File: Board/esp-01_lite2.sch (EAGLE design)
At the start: 26 parts, among them IC1 TINY13-20SU, K1 setup, K2 reset, X1 235-102, X2 235-102

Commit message: LED works, server ok, ESP 24h
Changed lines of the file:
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@@
 <grid distance="10" unitdist="mil" unit="mil" style="lines" multiple="1" display="no" altdistance="0.01" altunitdist="inch" altunit="inch"/>
 <layers>
-<layer number="1" name="Top" color="4" fill="1" visible="no" active="no"/>
-<layer number="2" name="Route2" color="1" fill="3" visible="no" active="no"/>
-<layer number="3" name="Route3" color="4" fill="3" visible="no" active="no"/>
-<layer number="4" name="Route4" color="1" fill="4" visible="no" active="no"/>
-<layer number="5" name="Route5" color="4" fill="4" visible="no" active="no"/>
-<layer number="6" name="Route6" color="1" fill="8" visible="no" active="no"/>
-<layer number="7" name="Route7" color="4" fill="8" visible="no" active="no"/>
-<layer number="8" name="Route8" color="1" fill="2" visible="no" active="no"/>
-<layer number="9" name="Route9" color="4" fill="2" visible="no" active="no"/>
-<layer number="10" name="Route10" color="1" fill="7" visible="no" active="no"/>
-<layer number="11" name="Route11" color="4" fill="7" visible="no" active="no"/>
-<layer number="12" name="Route12" color="1" fill="5" visible="no" active="no"/>
-<layer number="13" name="Route13" color="4" fill="5" visible="no" active="no"/>
-<layer number="14" name="Route14" color="1" fill="6" visible="no" active="no"/>
-<layer number="15" name="Route15" color="4" fill="6" visible="no" active="no"/>
-<layer number="16" name="Bottom" color="1" fill="1" visible="no" active="no"/>
-<layer number="17" name="Pads" color="2" fill="1" visible="no" active="no"/>
-<layer number="18" name="Vias" color="2" fill="1" visible="no" active="no"/>
-<layer number="19" name="Unrouted" color="6" fill="1" visible="no" active="no"/>
-<layer number="20" name="Dimension" color="15" fill="1" visible="no" active="no"/>
-<layer number="21" name="tPlace" color="7" fill="1" visible="no" active="no"/>
-<layer number="22" name="bPlace" color="7" fill="1" visible="no" active="no"/>
-<layer number="23" name="tOrigins" color="15" fill="1" visible="no" active="no"/>
-<layer number="24" name="bOrigins" color="15" fill="1" visible="no" active="no"/>
-<layer number="25" name="tNames" color="7" fill="1" visible="no" active="no"/>
-<layer number="26" name="bNames" color="7" fill="1" visible="no" active="no"/>
-<layer number="27" name="tValues" color="7" fill="1" visible="no" active="no"/>
-<layer number="28" name="bValues" color="7" fill="1" visible="no" active="no"/>
+<layer number="1" name="Top" color="4" fill="1" visible="yes" active="no"/>
+<layer number="2" name="Route2" color="1" fill="3" visible="yes" active="no"/>
+<layer number="3" name="Route3" color="4" fill="3" visible="yes" active="no"/>
+<layer number="4" name="Route4" color="1" fill="4" visible="yes" active="no"/>
+<layer number="5" name="Route5" color="4" fill="4" visible="yes" active="no"/>
+<layer number="6" name="Route6" color="1" fill="8" visible="yes" active="no"/>
+<layer number="7" name="Route7" color="4" fill="8" visible="yes" active="no"/>
+<layer number="8" name="Route8" color="1" fill="2" visible="yes" active="no"/>
+<layer number="9" name="Route9" color="4" fill="2" visible="yes" active="no"/>
+<layer number="10" name="Route10" color="1" fill="7" visible="yes" active="no"/>
+<layer number="11" name="Route11" color="4" fill="7" visible="yes" active="no"/>
+<layer number="12" name="Route12" color="1" fill="5" visible="yes" active="no"/>
+<layer number="13" name="Route13" color="4" fill="5" visible="yes" active="no"/>
+<layer number="14" name="Route14" color="1" fill="6" visible="yes" active="no"/>
+<layer number="15" name="Route15" color="4" fill="6" visible="yes" active="no"/>
+<layer number="16" name="Bottom" color="1" fill="1" visible="yes" active="no"/>
+<layer number="17" name="Pads" color="2" fill="1" visible="yes" active="no"/>
+<layer number="18" name="Vias" color="2" fill="1" visible="yes" active="no"/>
+<layer number="19" name="Unrouted" color="6" fill="1" visible="yes" active="no"/>
+<layer number="20" name="Dimension" color="15" fill="1" visible="yes" active="no"/>
+<layer number="21" name="tPlace" color="7" fill="1" visible="yes" active="no"/>
+<layer number="22" name="bPlace" color="7" fill="1" visible="yes" active="no"/>
+<layer number="23" name="tOrigins" color="15" fill="1" visible="yes" active="no"/>
+<layer number="24" name="bOrigins" color="15" fill="1" visible="yes" active="no"/>
+<layer number="25" name="tNames" color="7" fill="1" visible="yes" active="no"/>
+<layer number="26" name="bNames" color="7" fill="1" visible="yes" active="no"/>
+<layer number="27" name="tValues" color="7" fill="1" visible="yes" active="no"/>
+<layer number="28" name="bValues" color="7" fill="1" visible="yes" active="no"/>
 <layer number="29" name="tStop" color="7" fill="3" visible="no" active="no"/>
 <layer number="30" name="bStop" color="7" fill="6" visible="no" active="no"/>
@@
 <layer number="35" name="tGlue" color="7" fill="4" visible="no" active="no"/>
 <layer number="36" name="bGlue" color="7" fill="5" visible="no" active="no"/>
-<layer number="37" name="tTest" color="7" fill="1" visible="no" active="no"/>
-<layer number="38" name="bTest" color="7" fill="1" visible="no" active="no"/>
+<layer number="37" name="tTest" color="7" fill="1" visible="yes" active="no"/>
+<layer number="38" name="bTest" color="7" fill="1" visible="yes" active="no"/>
 <layer number="39" name="tKeepout" color="4" fill="11" visible="no" active="no"/>
 <layer number="40" name="bKeepout" color="1" fill="11" visible="no" active="no"/>
@@
 <layer number="44" name="Drills" color="7" fill="1" visible="no" active="no"/>
 <layer number="45" name="Holes" color="7" fill="1" visible="no" active="no"/>
-<layer number="46" name="Milling" color="3" fill="1" visible="no" active="no"/>
-<layer number="47" name="Measures" color="7" fill="1" visible="no" active="no"/>
-<layer number="48" name="Document" color="7" fill="1" visible="no" active="no"/>
-<layer number="49" name="Reference" color="7" fill="1" visible="no" active="no"/>
-<layer number="50" name="dxf" color="7" fill="1" visible="no" active="no"/>
-<layer number="51" name="tDocu" color="7" fill="1" visible="no" active="no"/>
-<layer number="52" name="bDocu" color="7" fill="1" visible="no" active="no"/>
-<layer number="53" name="tGND_GNDA" color="7" fill="9" visible="no" active="no"/>
-<layer number="54" name="bGND_GNDA" color="1" fill="9" visible="no" active="no"/>
-<layer number="56" name="wert" color="7" fill="1" visible="no" active="no"/>
-<layer number="57" name="tCAD" color="7" fill="1" visible="no" active="no"/>
+<layer number="46" name="Milling" color="3" fill="1" visible="yes" active="no"/>
+<layer number="47" name="Measures" color="7" fill="1" visible="yes" active="no"/>
+<layer number="48" name="Document" color="7" fill="1" visible="yes" active="no"/>
+<layer number="49" name="Reference" color="7" fill="1" visible="yes" active="no"/>
+<layer number="50" name="dxf" color="7" fill="1" visible="yes" active="no"/>
+<layer number="51" name="tDocu" color="7" fill="1" visible="yes" active="no"/>
+<layer number="52" name="bDocu" color="7" fill="1" visible="yes" active="no"/>
+<layer number="53" name="tGND_GNDA" color="7" fill="9" visible="yes" active="no"/>
+<layer number="54" name="bGND_GNDA" color="1" fill="9" visible="yes" active="no"/>
+<layer number="56" name="wert" color="7" fill="1" visible="yes" active="no"/>
+<layer number="57" name="tCAD" color="7" fill="1" visible="yes" active="no"/>
 <layer number="90" name="Modules" color="5" fill="1" visible="yes" active="yes"/>
 <layer number="91" name="Nets" color="2" fill="1" visible="yes" active="yes"/>
@@
 <attribute name="VALUE" x="140.208" y="110.49" size="1.778" layer="96" rot="R180"/>
 </instance>
-<instance part="SJ1" gate="1" x="61.214" y="30.734" rot="R180"/>
+<instance part="SJ1" gate="1" x="61.214" y="30.734" smashed="yes" rot="R180">
+<attribute name="NAME" x="63.754" y="28.194" size="1.778" layer="95" rot="R180"/>
+<attribute name="VALUE" x="63.754" y="34.544" size="1.778" layer="96" rot="R180"/>
+</instance>
 <instance part="GND4" gate="1" x="66.294" y="23.114" smashed="yes">
 <attribute name="VALUE" x="63.754" y="20.574" size="1.778" layer="96"/>

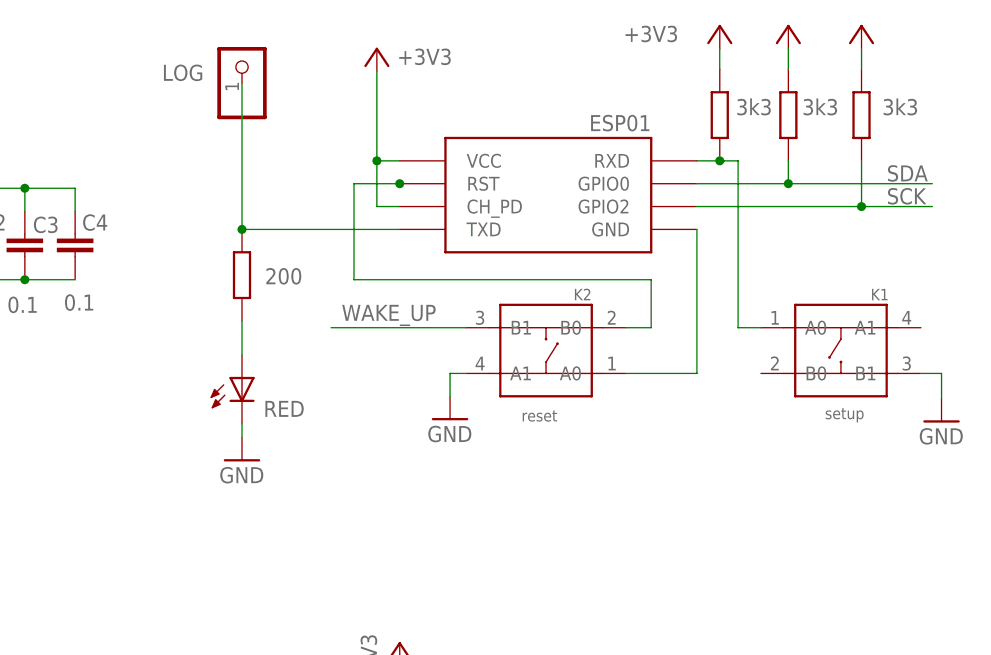
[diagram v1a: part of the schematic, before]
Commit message: new board
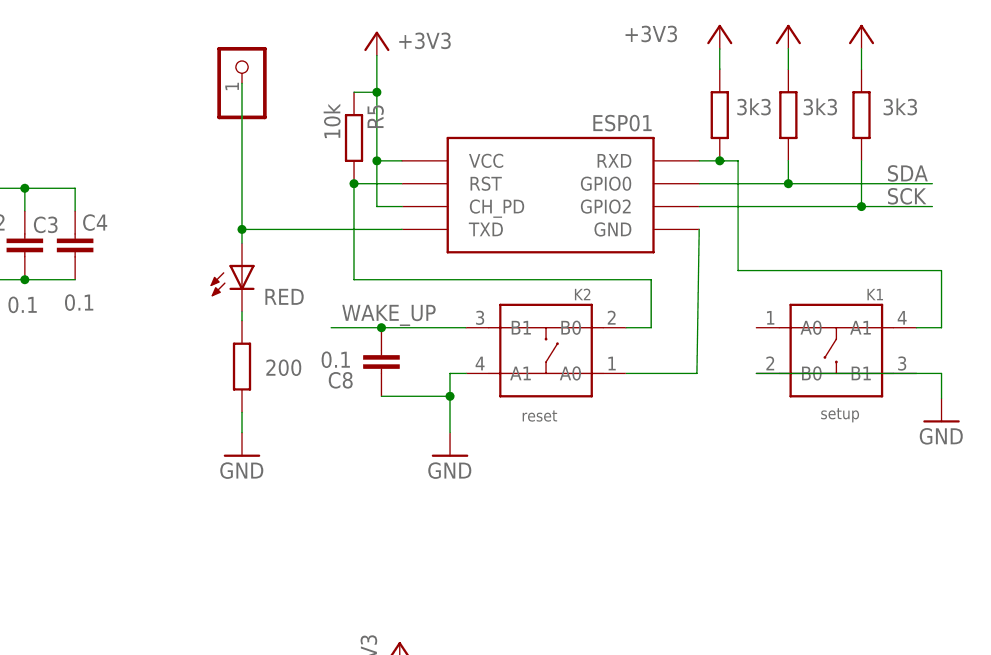
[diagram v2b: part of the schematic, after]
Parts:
- added C8: 0.1, resistor:C-EUC0805
- added R5: 10k, rcl:R-EU_R0805
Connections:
- removed net LOG: LOG.1, R4.1, U$1.TXD
- removed net N$12: LED1.A, R4.2
- new net N$1: LED1.A, LOG.1, U$1.TXD
- new net N$6: LED1.C, R4.1
- net +3V3: now also R5.1
- net GND: now also C8.1, K1.B0, R4.2; no longer LED1.C
- net N$2: now also R5.2
- net RX: now also K1.A1; no longer K1.A0
- net WAKE_UP: now also C8.2
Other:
- moved on the sheet: K1

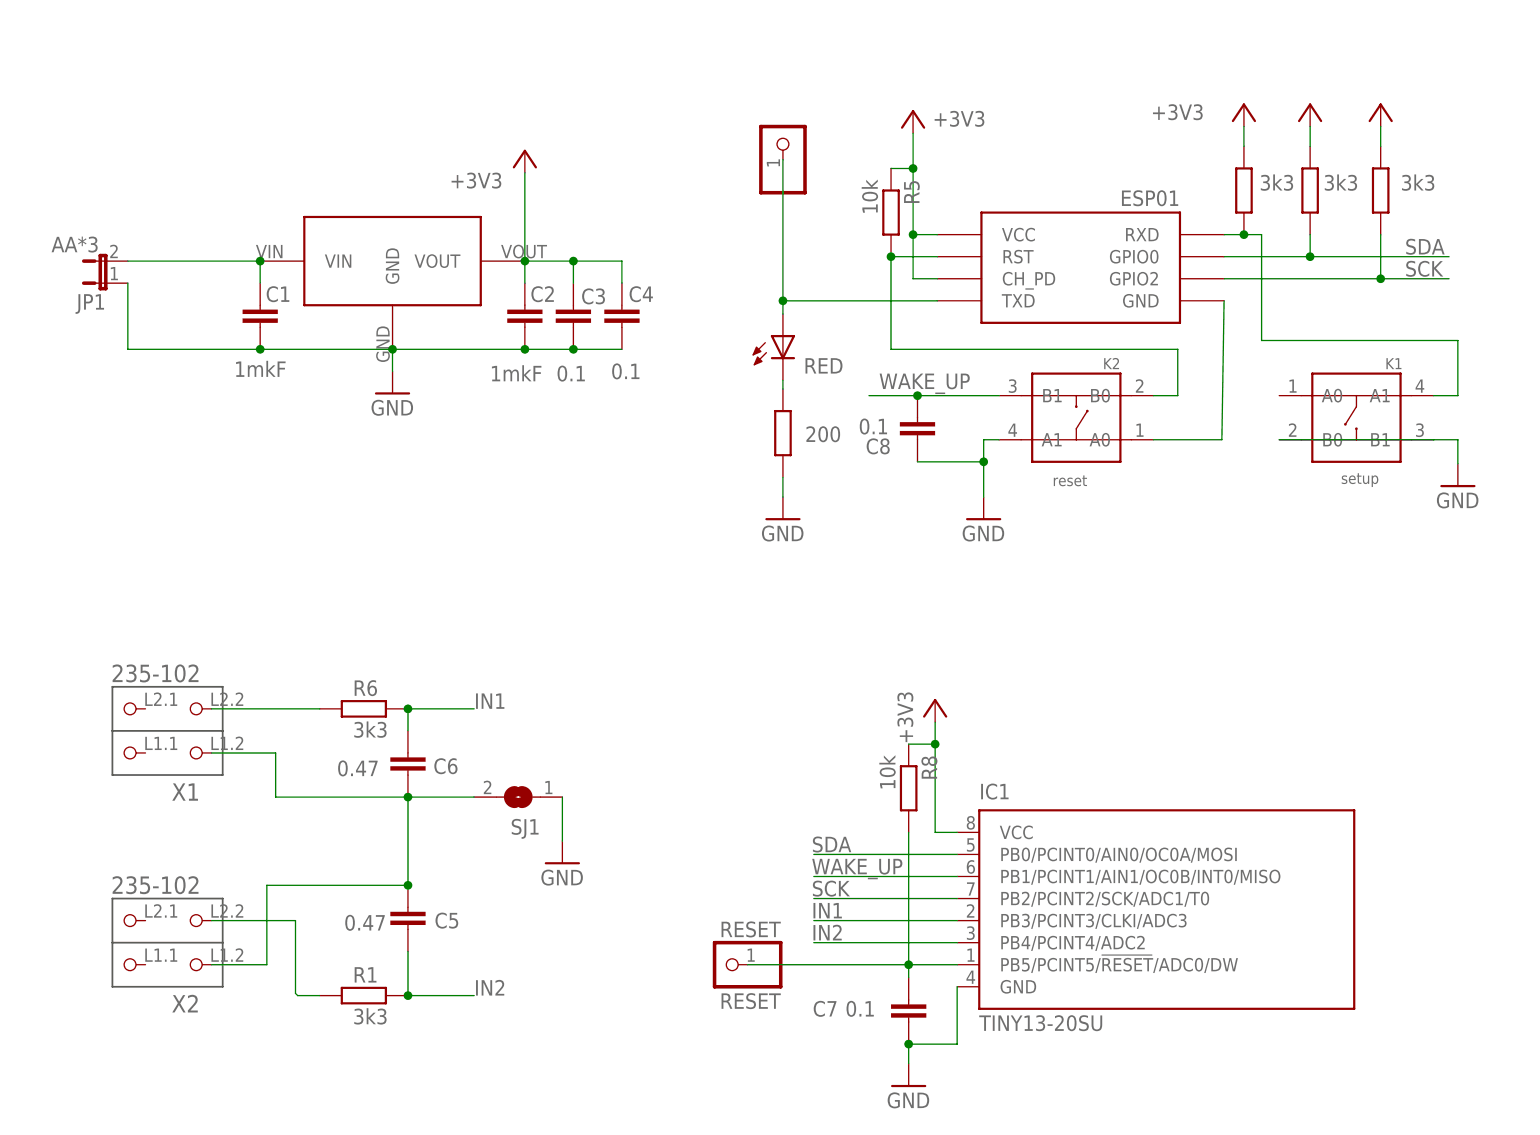
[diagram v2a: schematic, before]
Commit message: board for one_button
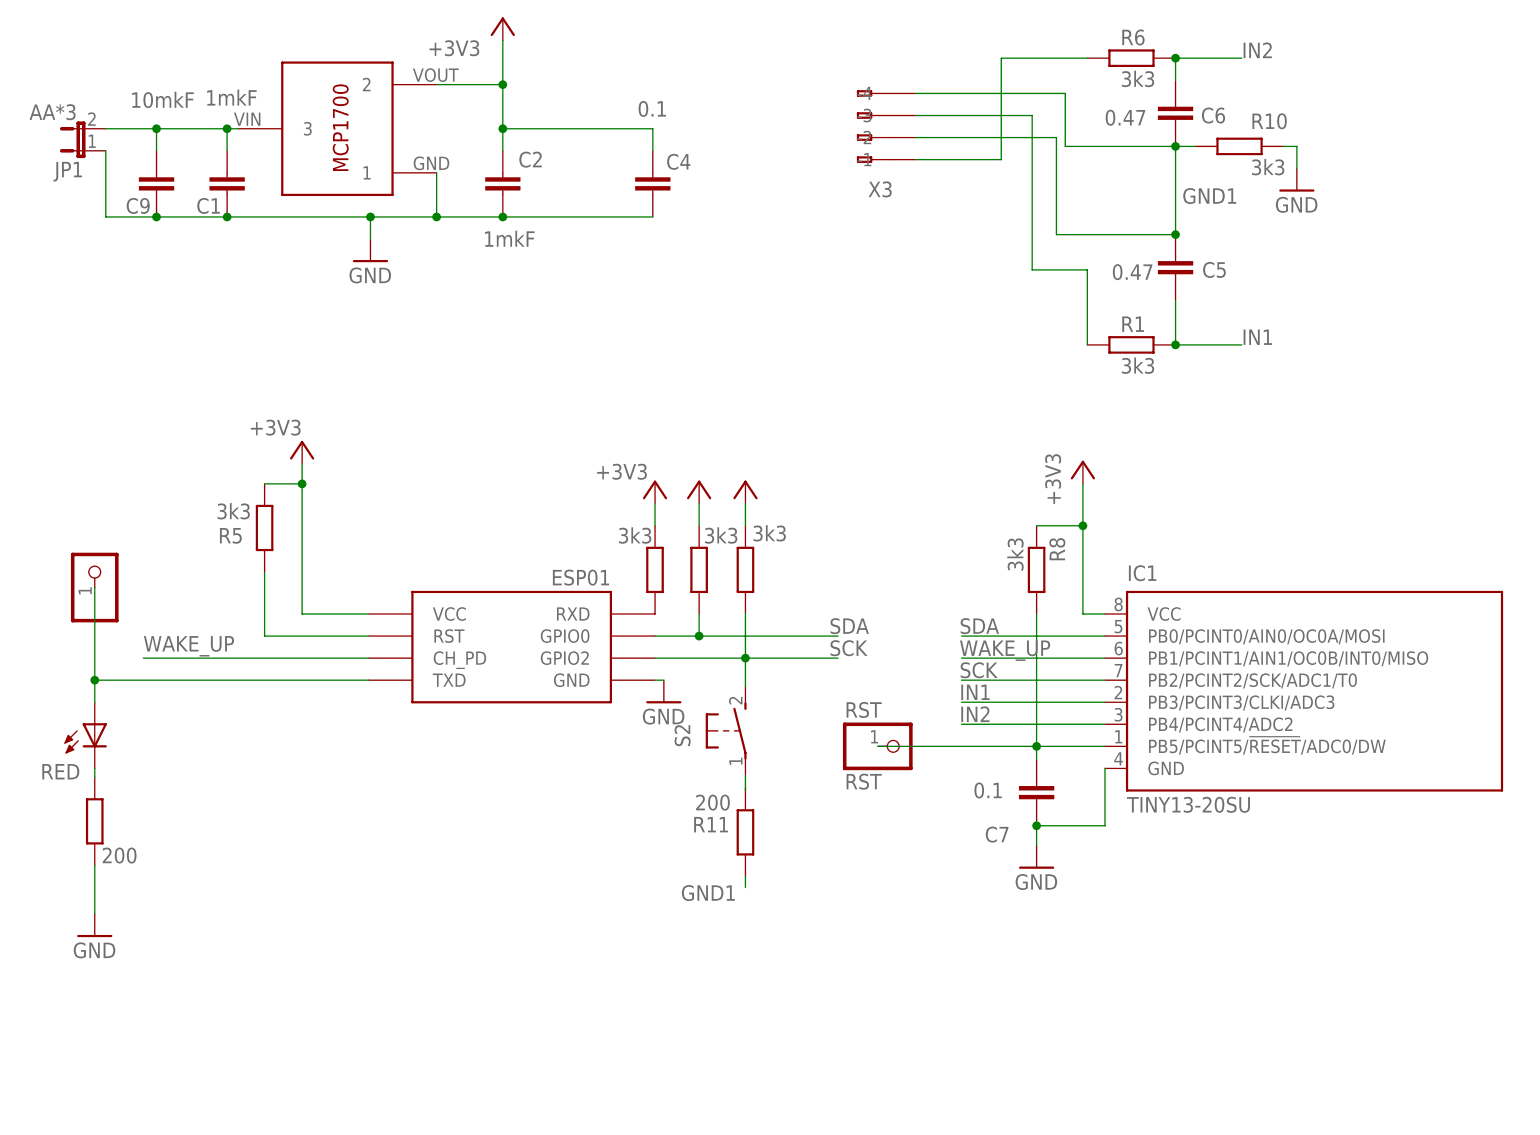
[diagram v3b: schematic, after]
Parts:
- removed C3, C8: 0.1, resistor:C-EUC0805
- removed K1: setup, Seeed-OPL-Button:DIP-BUTTON-4P
- removed K2: reset, Seeed-OPL-Button:DIP-BUTTON-4P
- removed RESET: RESET, pinhead:PINHD-1X1
- removed SJ1: (no value), jumper:SJ
- removed X1, X2: 235-102, con-wago_235:235-102
- added C9: 10mkF, rcl:C-EU025-030X050
- added R10: 3k3, resistor:R-EU_M0805
- added R11: 200, rcl:R-EU_R0805
- added RST: RST, pinhead:PINHD-1X1
- added S2: (no value), switch-omron:31-XX
- added X3: (no value), con-wago255:233-104
- C4: device resistor:C-EU050-024X044 -> rcl:C-EUC0805
- R3: device resistor:R-EU_0207/5V -> rcl:R-EU_R0805
- R4: device resistor:R-EU_0207/5V -> rcl:R-EU_0207/2V
- R5: value 10k -> 3k3
- R8: value 10k -> 3k3; device rcl:R-EU_R0805 -> rcl:R-EU_0204/5
- U$2: value HT7333 -> MCP1700T-3302E/TT; device HT7333_SOT89:HT7333 -> MCP1700T-3302E_TT:MCP1700T-3302E/TT
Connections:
- removed net N$5: C5.1, C6.1, SJ1.2, X1.P1.2, X2.P1.2
- new net N$11: R5.2, U$1.RST
- net +3V3: now also C2.1, U$2.2; no longer C2.2, C3.2, U$1.CH_PD, U$2.VOUT
- net AA*3: now also C1.1, C9.1, U$2.3; no longer C1.2, U$2.VIN
- net GND: now also C1.2, C2.2, C9.2, R10.2, U$1.GND, U$2.1; no longer C1.1, C2.1, C3.1, C8.1, K1.B0, K1.B1, K2.A1, SJ1.1, U$2.GND
- net GND1: now also C5.1, C6.1, R10.1, R11.2, X3.-2, X3.-4; no longer K2.A0, U$1.GND
- net IN1: now also C5.2, R1.2; no longer C6.2, R6.2
- net IN2: now also C6.2, R6.2; no longer C5.2, R1.2
- net N$13: now also RST.1; no longer RESET.1
- net N$2: now also R11.1, S2.P; no longer K2.B0, R5.2, U$1.RST
- net N$3: now also X3.-1; no longer X1.P2.2
- net N$4: now also X3.-3; no longer X2.P2.2
- net RX: no longer K1.A1
- net SCK: now also S2.S
- net WAKE_UP: now also U$1.CH_PD; no longer C8.2, K2.B1
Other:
- moved on the sheet: C1, C2, C4, C5, C6, C7, IC1, JP1, R1, R5, R6, R8
